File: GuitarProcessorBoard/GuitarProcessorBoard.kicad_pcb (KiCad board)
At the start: 4 copper layers, 86 x 65 mm, 126 parts, among them J301 SWD Header, J302 PWR, J304 MODE, J305 BYP, J307 ScopeGroundLoop, SW301 RST, SW302 BOOT, U1 AMS1117, U201 TLV320AIC3204, U202 TL074, U301 STM32H7B0VBT6, U302 TPS63070, U303 SSD1306_OLED_128x64, U304 74HC595, Y301 32MHz, Y302 32.768kHZ

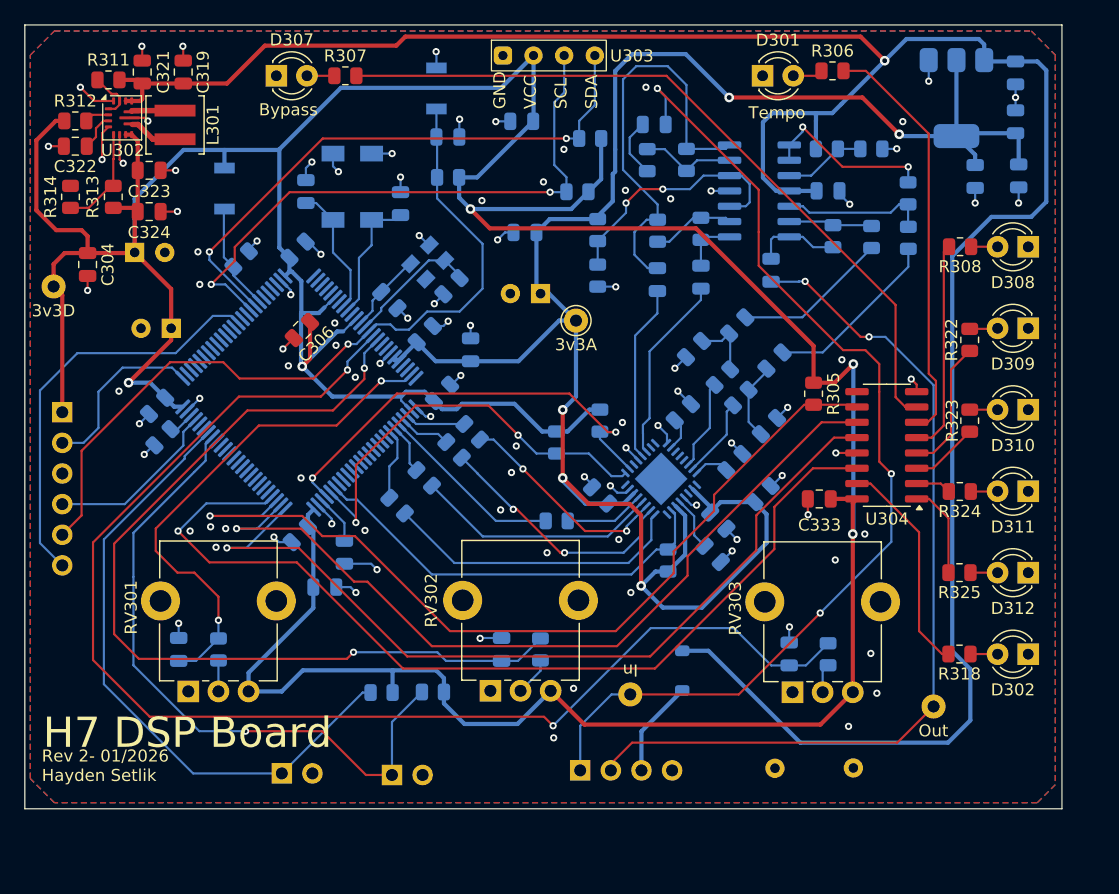
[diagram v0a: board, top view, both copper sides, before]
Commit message: new layout
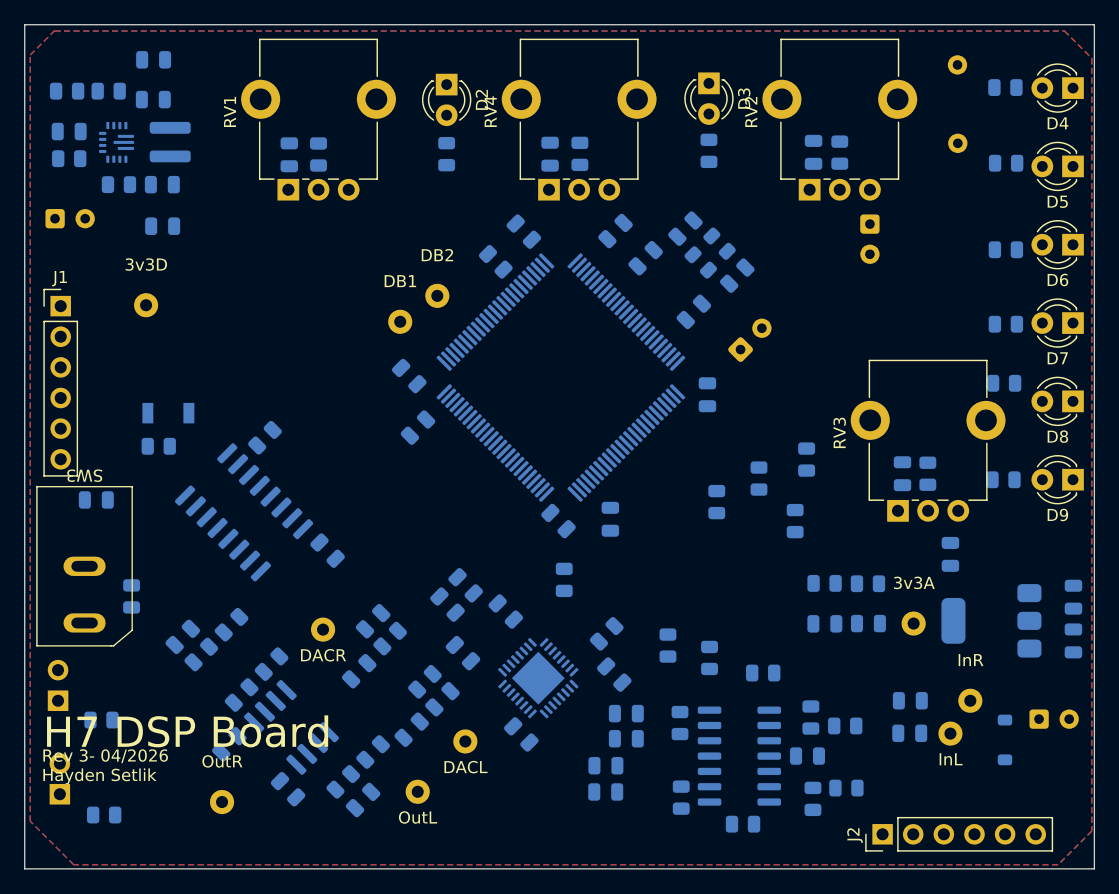
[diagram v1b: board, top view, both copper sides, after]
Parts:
- removed C201, C208, C209, C210, C211, C214, C215, C216, C304, C306, C307, C309, C311, C312, C313, C318, C322, C332, C333: 100n, Capacitor_SMD:C_0805_2012Metric
- removed C202, C308, C310, C314: 2u2, Capacitor_SMD:C_0805_2012Metric
- removed C203, C204, C205, C206, C303, C319, C321, C323: 10u, Capacitor_SMD:C_0805_2012Metric
- removed C207, C212: 4n7, Capacitor_SMD:C_0805_2012Metric
- removed C301, C302: 10p, Capacitor_SMD:C_0805_2012Metric
- removed C315, C317: 6p, Capacitor_SMD:C_0805_2012Metric
- removed C324: 22u, Capacitor_SMD:C_0805_2012Metric
- removed C326: 330u, Capacitor_THT:CP_Radial_D5.0mm_P2.50mm
- removed C327, C328, C329: 10n, Capacitor_SMD:C_0805_2012Metric
- removed D301: RED, LED_THT:LED_D3.0mm
- removed D302, D308, D309, D310, D311, D312: ORANGE, LED_THT:LED_D3.0mm
- removed D304: PMEG3030, Diode_SMD:D_SOD-123
- removed D307: GREEN, LED_THT:LED_D3.0mm
- removed J301: SWD Header, Connector_PinHeader_2.54mm:PinHeader_1x06_P2.54mm_Vertical
- removed J302: PWR, Connector_PinHeader_2.54mm:PinHeader_1x04_P2.54mm_Vertical
- removed J304: MODE, Connector_PinHeader_2.54mm:PinHeader_1x02_P2.54mm_Vertical
- removed J305: BYP, Connector_PinHeader_2.54mm:PinHeader_1x02_P2.54mm_Vertical
- removed J307: ScopeGroundLoop, Connector:THT_GND_WIRE
- removed L301: 1u5, Inductor_SMD:L_Coilcraft_XAL4020-XXX
- removed R201, R305, R313: 47k, Resistor_SMD:R_0805_2012Metric
- removed R202, R203, R205, R209, R210, R211, R215, R309, R310, R312, R327, R328: 100k, Resistor_SMD:R_0805_2012Metric
- removed R204, R212, R216: 51k, Resistor_SMD:R_0805_2012Metric
- removed R206, R207: 470k, Resistor_SMD:R_0805_2012Metric
- removed R208, R214: 1k, Resistor_SMD:R_0805_2012Metric
- removed R220, R330, R331, R332, R333: 22, Resistor_SMD:R_0805_2012Metric
- removed R301, R302, R303, R304: 2k2, Resistor_SMD:R_0805_2012Metric
- removed R306, R307, R308, R318, R322, R323, R324, R325: 470, Resistor_SMD:R_0805_2012Metric
- removed R311: 10k, Resistor_SMD:R_0805_2012Metric
- removed R314: 5k1, Resistor_SMD:R_0805_2012Metric
- removed R315, R316, R317: 22k, Resistor_SMD:R_0805_2012Metric
- removed RV301, RV302, RV303: 100kB, Potentiometer_THT:Potentiometer_Alpha_RD901F-40-00D_Single_Vertical_CircularHoles
- removed SW301: RST, Button_Switch_SMD:SW_SPST_B3U-1000P
- removed SW302: BOOT, Button_Switch_SMD:SW_SPST_B3U-1000P
- removed TP301: In, TestPoint:TestPoint_THTPad_D2.0mm_Drill1.0mm_VAL
- removed TP302: Out, TestPoint:TestPoint_THTPad_D2.0mm_Drill1.0mm_VAL
- removed TP303: 3v3D, TestPoint:TestPoint_THTPad_D2.0mm_Drill1.0mm_VAL
- removed U201: TLV320AIC3204, Package_DFN_QFN:VQFN-32-1EP_5x5mm_P0.5mm_EP3.1x3.1mm
- removed U202: TL074, Package_SO:SOIC-14_3.9x8.7mm_P1.27mm
- removed U301: STM32H7B0VBT6, Package_QFP:LQFP-100_14x14mm_P0.5mm
- removed U302: TPS63070, Package_DFN_QFN:TXN_QFN15
- removed U303: SSD1306_OLED_128x64, Display:SSD1306_OLED_128x64_OffBoard
- removed U304: 74HC595, Package_SO:SOIC-16_3.9x9.9mm_P1.27mm
- removed Y301: 32MHz, Crystal:Crystal_SMD_EuroQuartz_MT-4Pin_3.2x2.5mm
- removed Y302: 32.768kHZ, Crystal:Crystal_SMD_SeikoEpson_MC306-4Pin_8.0x3.2mm
- added C10: 10u, Capacitor_SMD:C_0805_2012Metric, B.Cu at (-142.6, 83.1)
- added C11: 10u, Capacitor_SMD:C_0805_2012Metric, B.Cu at (-142.4, 77.5)
- added C12: 10u, Capacitor_SMD:C_0805_2012Metric, B.Cu at (-165.9, 81.7)
- added C13: 10u, Capacitor_SMD:C_0805_2012Metric, B.Cu at (-137.8, 89.8)
- added C14: 100n, Capacitor_SMD:C_0805_2012Metric, B.Cu at (-143.9, 79.0)
- added C15: 4n7, Capacitor_SMD:C_0805_2012Metric, B.Cu at (-150.1, 80.4)
- added C16: 4n7, Capacitor_SMD:C_0805_2012Metric, B.Cu at (-144.3, 86.9)
- added C17: 2u2, Capacitor_SMD:C_0805_2012Metric, B.Cu at (-139.1, 79.6)
- added C18: 100n, Capacitor_SMD:C_0805_2012Metric, B.Cu at (-146.9, 89.4)
- added C19: 100n, Capacitor_SMD:C_0805_2012Metric, B.Cu at (-151.2, 84.6)
- added C20: 10u, Capacitor_SMD:C_0805_2012Metric, B.Cu at (-130.1, 84.8)
- added C21: 1u, Capacitor_SMD:C_0805_2012Metric, B.Cu at (-150.9, 95.3)
- added C22: 1u, Capacitor_SMD:C_0805_2012Metric, B.Cu at (-162.0, 90.6)
- added C24: 10p, Capacitor_SMD:C_0805_2012Metric, B.Cu at (-119.9, 51.8)
- added C25: 10u, Capacitor_SMD:C_0805_2012Metric, B.Cu at (-173.0, 70.4)
- added C26: 10p, Capacitor_SMD:C_0805_2012Metric, B.Cu at (-124.2, 47.9)
- added C27: 100n, Capacitor_SMD:C_0805_2012Metric, B.Cu at (-153.8, 74.6)
- added C28: 100n, Capacitor_SMD:C_0805_2012Metric, B.Cu at (-127.5, 50.3)
- added C29: 100n, Capacitor_SMD:C_0805_2012Metric, B.Cu at (-130.0, 48.1)
- added C30: 100n, Capacitor_SMD:C_0805_2012Metric, B.Cu at (-147.1, 60.1)
- added C31: 2u2, Capacitor_SMD:C_0805_2012Metric, B.Cu at (-130.4, 72.0)
- added C32: 100n, Capacitor_SMD:C_0805_2012Metric, B.Cu at (-134.7, 72.1)
- added C33: 2u2, Capacitor_SMD:C_0805_2012Metric, B.Cu at (-146.3, 64.4)
- added C34: 100n, Capacitor_SMD:C_0805_2012Metric, B.Cu at (-122.3, 61.6)
- added C35: 100n, Capacitor_SMD:C_0805_2012Metric, B.Cu at (-137.6, 48.1)
- added C36: 100n, Capacitor_SMD:C_0805_2012Metric, B.Cu at (-123.5, 54.8)
- added C37: 330u, Capacitor_THT:CP_Radial_D5.0mm_P2.50mm, B.Cu at (-94.8, 88.5)
- added C40: 100n, Capacitor_SMD:C_0805_2012Metric, B.Cu at (-92.0, 82.1)
- added C41: 330u, Capacitor_THT:CP_Radial_D5.0mm_P2.50mm, B.Cu at (-119.6, 57.9)
- added C42: 100n, Capacitor_SMD:C_0805_2012Metric, B.Cu at (-92.0, 78.4)
- added C43: 1u, Capacitor_SMD:C_0805_2012Metric, B.Cu at (-109.0, 80.6)
- added C44: 10u, Capacitor_SMD:C_0805_2012Metric, B.Cu at (-102.2, 74.9)
- added C45: 10n, Capacitor_SMD:C_0805_2012Metric, B.Cu at (-157.0, 41.8)
- added C46: 10n, Capacitor_SMD:C_0805_2012Metric, B.Cu at (-113.5, 41.5)
- added C47: 10u, Capacitor_SMD:C_0805_2012Metric, B.Cu at (-167.5, 47.7)
- added C48: 10n, Capacitor_SMD:C_0805_2012Metric, B.Cu at (-106.2, 68.2)
- added C49: 10n, Capacitor_SMD:C_0805_2012Metric, B.Cu at (-135.4, 41.7)
- added C50: 10u, Capacitor_SMD:C_0805_2012Metric, B.Cu at (-167.6, 44.2)
- added C51: 100n, Capacitor_SMD:C_0805_2012Metric, B.Cu at (-175.3, 39.8)
- added C53: 10u, Capacitor_SMD:C_0805_2012Metric, B.Cu at (-168.3, 37.2)
- added C54: 22u, Capacitor_SMD:C_0805_2012Metric, B.Cu at (-168.3, 33.9)
- added C55: 330u, Capacitor_THT:CP_Radial_D5.0mm_P2.50mm, B.Cu at (-176.4, 47.0)
- added C56: 330u, Capacitor_THT:CP_Radial_D5.0mm_P2.50mm, B.Cu at (-108.9, 47.5)
- added C8: 100n, Capacitor_SMD:C_0805_2012Metric, B.Cu at (-114.0, 91.6)
- added C9: 10u, Capacitor_SMD:C_0805_2012Metric, B.Cu at (-112.6, 80.6)
- added D1: PMEG3030, Diode_SMD:D_SOD-123, B.Cu at (-97.7, 90.3)
- added D2: RED, LED_THT:LED_D3.0mm, F.Cu at (-144.0, 35.9)
- added D3: GREEN, LED_THT:LED_D3.0mm, F.Cu at (-122.2, 35.8)
- added D4: ORANGE, LED_THT:LED_D3.0mm, F.Cu at (-92.0, 36.2)
- added D5: ORANGE, LED_THT:LED_D3.0mm, F.Cu at (-92.0, 42.7)
- added D6: ORANGE, LED_THT:LED_D3.0mm, F.Cu at (-92.0, 49.2)
- added D7: ORANGE, LED_THT:LED_D3.0mm, F.Cu at (-92.0, 55.7)
- added D8: ORANGE, LED_THT:LED_D3.0mm, F.Cu at (-92.0, 62.2)
- added D9: ORANGE, LED_THT:LED_D3.0mm, F.Cu at (-92.0, 68.7)
- added J1: SWD Header, Connector_PinHeader_2.54mm:PinHeader_1x06_P2.54mm_Vertical, F.Cu at (-176.0, 54.3)
- added J2: IO, Connector_PinHeader_2.54mm:PinHeader_1x06_P2.54mm_Vertical, F.Cu at (-107.8, 98.1)
- added J3: ScopeGroundLoop, Capacitor_THT:THT_GND_WIRE, B.Cu at (-101.6, 37.4)
- added J4: MODE, Connector_PinHeader_2.54mm:PinHeader_1x02_P2.54mm_Vertical, B.Cu at (-176.1, 94.8)
- added J5: BYP, Connector_PinHeader_2.54mm:PinHeader_1x02_P2.54mm_Vertical, B.Cu at (-176.2, 87.0)
- added L1: 1u5, Inductor_SMD:L_Coilcraft_XAL4020-XXX, B.Cu at (-166.9, 40.7)
- added R1: 470k, Resistor_SMD:R_0805_2012Metric, B.Cu at (-117.7, 84.7)
- added R10: 22, Resistor_SMD:R_0805_2012Metric, B.Cu at (-130.7, 81.5)
- added R11: 100k, Resistor_SMD:R_0805_2012Metric, B.Cu at (-109.0, 77.3)
- added R12: 100k, Resistor_SMD:R_0805_2012Metric, B.Cu at (-112.6, 77.3)
- added R13: 100k, Resistor_SMD:R_0805_2012Metric, B.Cu at (-164.3, 83.2)
- added R14: 100k, Resistor_SMD:R_0805_2012Metric, B.Cu at (-161.8, 80.7)
- added R15: 1k, Resistor_SMD:R_0805_2012Metric, B.Cu at (-148.7, 81.9)
- added R16: 1k, Resistor_SMD:R_0805_2012Metric, B.Cu at (-145.8, 85.5)
- added R17: 470k, Resistor_SMD:R_0805_2012Metric, B.Cu at (-150.1, 91.3)
- added R18: 470k, Resistor_SMD:R_0805_2012Metric, B.Cu at (-158.5, 84.0)
- added R19: 470k, Resistor_SMD:R_0805_2012Metric, B.Cu at (-152.6, 93.8)
- added R2: 470k, Resistor_SMD:R_0805_2012Metric, B.Cu at (-110.9, 89.1)
- added R20: 470k, Resistor_SMD:R_0805_2012Metric, B.Cu at (-161.0, 86.5)
- added R21: 100k, Resistor_SMD:R_0805_2012Metric, B.Cu at (-167.8, 65.9)
- added R22: 100k, Resistor_SMD:R_0805_2012Metric, B.Cu at (-139.9, 50.6)
- added R23: 47k, Resistor_SMD:R_0805_2012Metric, B.Cu at (-159.0, 65.2)
- added R26: 22, Resistor_SMD:R_0805_2012Metric, B.Cu at (-121.6, 70.5)
- added R27: 22, Resistor_SMD:R_0805_2012Metric, B.Cu at (-114.1, 67.0)
- added R28: 22, Resistor_SMD:R_0805_2012Metric, B.Cu at (-118.1, 68.6)
- added R29: 22, Resistor_SMD:R_0805_2012Metric, B.Cu at (-115.1, 72.1)
- added R3: 470k, Resistor_SMD:R_0805_2012Metric, B.Cu at (-119.4, 97.3)
- added R30: 2k2, Resistor_SMD:R_0805_2012Metric, B.Cu at (-125.6, 82.5)
- added R31: 2k2, Resistor_SMD:R_0805_2012Metric, B.Cu at (-122.2, 83.5)
- added R32: 100k, Resistor_SMD:R_0805_2012Metric, B.Cu at (-172.4, 96.5)
- added R33: 100k, Resistor_SMD:R_0805_2012Metric, B.Cu at (-172.6, 88.6)
- added R34: 22k, Resistor_SMD:R_0805_2012Metric, B.Cu at (-154.6, 41.7)
- added R35: 22k, Resistor_SMD:R_0805_2012Metric, B.Cu at (-111.4, 41.6)
- added R36: 22k, Resistor_SMD:R_0805_2012Metric, B.Cu at (-104.1, 68.2)
- added R37: 22k, Resistor_SMD:R_0805_2012Metric, B.Cu at (-132.9, 41.7)
- added R38: 10k, Resistor_SMD:R_0805_2012Metric, B.Cu at (-171.2, 44.2)
- added R39: 47k, Resistor_SMD:R_0805_2012Metric, B.Cu at (-170.1, 78.4)
- added R4: 470k, Resistor_SMD:R_0805_2012Metric, B.Cu at (-110.8, 94.3)
- added R42: 100k, Resistor_SMD:R_0805_2012Metric, B.Cu at (-175.3, 42.1)
- added R43: 47k, Resistor_SMD:R_0805_2012Metric, B.Cu at (-172.0, 36.5)
- added R44: 15k, Resistor_SMD:R_0805_2012Metric, B.Cu at (-175.4, 36.5)
- added R45: 470, Resistor_SMD:R_0805_2012Metric, B.Cu at (-144.0, 41.7)
- added R46: 470, Resistor_SMD:R_0805_2012Metric, B.Cu at (-122.2, 41.4)
- added R47: 470, Resistor_SMD:R_0805_2012Metric, B.Cu at (-97.6, 36.2)
- added R48: 470, Resistor_SMD:R_0805_2012Metric, B.Cu at (-97.6, 42.5)
- added R49: 470, Resistor_SMD:R_0805_2012Metric, B.Cu at (-97.6, 49.6)
- added R5: 470k, Resistor_SMD:R_0805_2012Metric, B.Cu at (-124.6, 88.9)
- added R50: 470, Resistor_SMD:R_0805_2012Metric, B.Cu at (-97.6, 55.8)
- added R51: 470, Resistor_SMD:R_0805_2012Metric, B.Cu at (-97.8, 60.7)
- added R52: 470, Resistor_SMD:R_0805_2012Metric, B.Cu at (-97.8, 68.7)
- added R6: 470k, Resistor_SMD:R_0805_2012Metric, B.Cu at (-113.8, 88.4)
- added R7: 470k, Resistor_SMD:R_0805_2012Metric, B.Cu at (-124.5, 95.1)
- added R8: 470k, Resistor_SMD:R_0805_2012Metric, B.Cu at (-113.6, 95.2)
- added R9: 47k, Resistor_SMD:R_0805_2012Metric, B.Cu at (-134.2, 77.0)
- added RV1: 100kB, Potentiometer_THT:Potentiometer_Alpha_RD901F-40-00D_Single_Vertical_CircularHoles, F.Cu at (-157.1, 44.6)
- added RV2: 100kB, Potentiometer_THT:Potentiometer_Alpha_RD901F-40-00D_Single_Vertical_CircularHoles, F.Cu at (-113.9, 44.6)
- added RV3: 100kB, Potentiometer_THT:Potentiometer_Alpha_RD901F-40-00D_Single_Vertical_CircularHoles, F.Cu at (-106.5, 71.3)
- added RV4: 100kB, Potentiometer_THT:Potentiometer_Alpha_RD901F-40-00D_Single_Vertical_CircularHoles, F.Cu at (-135.5, 44.6)
- added SW1: RST, Button_Switch_SMD:SW_SPST_B3U-1000P, B.Cu at (-167.1, 63.2)
- added SW3: SW_1, Button_Switch_THT:MiniToggle_SPST, F.Cu at (-174.0, 75.9)
- added TP10: DACR, TestPoint:TestPoint_THTPad_D2.0mm_Drill1.0mm_VAL, B.Cu at (-154.2, 81.1)
- added TP2: InR, TestPoint:TestPoint_THTPad_D2.0mm_Drill1.0mm_VAL, B.Cu at (-100.5, 87.0)
- added TP3: 3v3D, TestPoint:TestPoint_THTPad_D2.0mm_Drill1.0mm_VAL, B.Cu at (-168.9, 54.2)
- added TP4: OutL, TestPoint:TestPoint_THTPad_D2.0mm_Drill1.0mm_VAL, B.Cu at (-146.4, 94.6)
- added TP5: OutR, TestPoint:TestPoint_THTPad_D2.0mm_Drill1.0mm_VAL, B.Cu at (-162.6, 95.4)
- added TP6: 3v3A, TestPoint:TestPoint_THTPad_D2.0mm_Drill1.0mm_VAL, B.Cu at (-105.2, 80.6)
- added TP7: DB1, TestPoint:TestPoint_THTPad_D2.0mm_Drill1.0mm_VAL, B.Cu at (-147.8, 55.6)
- added TP8: DB2, TestPoint:TestPoint_THTPad_D2.0mm_Drill1.0mm_VAL, B.Cu at (-144.8, 53.5)
- added TP9: DACL, TestPoint:TestPoint_THTPad_D2.0mm_Drill1.0mm_VAL, B.Cu at (-142.4, 90.4)
- added U2: TL072, Package_SO:SOIC-8_3.9x4.9mm_P1.27mm, B.Cu at (-156.8, 89.2)
- added U3: TLV320AIC3204, Package_DFN_QFN:VQFN-32-1EP_5x5mm_P0.5mm_EP3.1x3.1mm, B.Cu at (-136.4, 85.2)
- added U4: 74HC595, Package_SO:SOIC-16_3.9x9.9mm_P1.27mm, B.Cu at (-160.8, 71.4)
- added U5: STM32H7B0VBT6, Package_QFP:LQFP-100_14x14mm_P0.5mm, B.Cu at (-134.5, 60.2)
- added U6: AMS1117, Package_TO_SOT_SMD:SOT-223-3_TabPin2, B.Cu at (-98.8, 80.4)
- added U7: TPS63070, Converter_DCDC:TXN_QFN15, B.Cu at (-171.3, 40.7)
- added Y1: 32MHz, Crystal:Crystal_SMD_EuroQuartz_MT-4Pin_3.2x2.5mm, B.Cu at (-122.1, 49.9)
- C1, C3: value 330u -> 100n; footprint Capacitor_THT:CP_Radial_D5.0mm_P2.50mm -> Capacitor_SMD:C_0805_2012Metric
- C2, C7: value 10u -> 100n
- C6: value 1u -> 100n
- TP1: value 3v3A -> InL; moved to B.Cu
- U1: value AMS1117 -> TL074; footprint Package_TO_SOT_SMD:SOT-223-3_TabPin2 -> Package_SO:SOIC-14_3.9x8.7mm_P1.27mm
- moved C7 79.1 mm to (-157.1, 94.4), turned to -45 degrees
- moved C1 68.6 mm to (-105.5, 87.0)
- moved C5 63.3 mm to (-130.8, 92.4), turned to 180 degrees
- moved C4 62.2 mm to (-129.1, 88.1), turned to 180 degrees
- moved C6 59.5 mm to (-130.8, 94.6), turned to 180 degrees
- moved U1 57.5 mm to (-119.7, 91.6), turned to 180 degrees
- moved C2 52.4 mm to (-105.6, 89.7)
- moved TP1 46.2 mm to (-102.2, 89.8), turned to 180 degrees
- moved C3 37.6 mm to (-129.1, 90.2)
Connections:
- C1 pad 1: +3.3V -> IN_R
- C1 pad 2: GND -> Net-(C1-Pad2)
- C2 pad 1: +3.3VA -> IN_L
- C2 pad 2: GND -> Net-(C2-Pad2)
- C3 pad 1: +3.3VA -> /Audio/RightInputNeg
- C3 pad 2: GND -> /Audio/In1R
- C4 pad 1: GND -> /Audio/RightInputPos
- C4 pad 2: VCC -> /Audio/In1L
- C5 pad 1: GND -> /Audio/LeftInputNeg
- C5 pad 2: +3.3VA -> /Audio/In2L
- C6 pad 1: +3.3VA -> /Audio/LeftInputPos
- C6 pad 2: GND -> /Audio/In2R
- C7 pad 1: +3.3VA -> VCC
- TP1 pad 1: +3.3VA -> IN_L
- U1 pad 1: GND -> /Audio/RightInputPos
- U1 pad 2: +3.3VA -> Net-(U1A--)
- U1 pad 3: VCC -> /Audio/Bias1
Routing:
- net +3.3V: track 354.6 -> 0.00 mm, vias 5 -> 0
- net VCC: track 196.9 -> 0.00 mm, vias 1 -> 0
- net +3.3VA: track 161.5 -> 0.00 mm, vias 5 -> 0
- net ADC_C: track 109.1 -> 0.00 mm, vias 2 -> 0
- net GND: track 95.2 -> 0.00 mm, vias 98 -> 0
- net FX_IN: track 85.8 -> 0.00 mm, vias 3 -> 0
- net LED_DATA: track 79.0 -> 0.00 mm, vias 1 -> 0
- net ADC_B: track 75.1 -> 0.00 mm, vias 2 -> 0
- net LED_NRST: track 73.3 -> 0.00 mm, vias 1 -> 0
- net FX_OUT: track 73.0 -> 0.00 mm, vias 2 -> 0
- net LED_LATCH: track 71.3 -> 0.00 mm, vias 1 -> 0
- net LED_SCK: track 68.6 -> 0.00 mm, vias 1 -> 0
- net NRST: track 64.4 -> 0.00 mm, vias 1 -> 0
- net /MCU/LED_BYPASS: track 62.3 -> 0.00 mm
- net BYP_BTN: track 54.8 -> 0.00 mm, vias 1 -> 0
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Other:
- board size 86 x 65 mm -> 88.7 x 70 mm
- board text added: "INL"
- board text added: "INR"
- board text added: "OUTL"
- board text added: "OUTR"
- board text added: "Rev 3- 04/2026 Hayden Setlik"
- board text removed: "Bypass"
- board text removed: "IN"
- board text removed: "OUT"
- board text removed: "Rev 2- 01/2026 Hayden Setlik"
- board text removed: "Tempo"
